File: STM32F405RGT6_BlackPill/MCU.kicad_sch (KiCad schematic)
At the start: 31 parts, among them J1 Conn_01x04, U1 STM32F405RGTx, Y1 25Mhz, Y2 Crystal

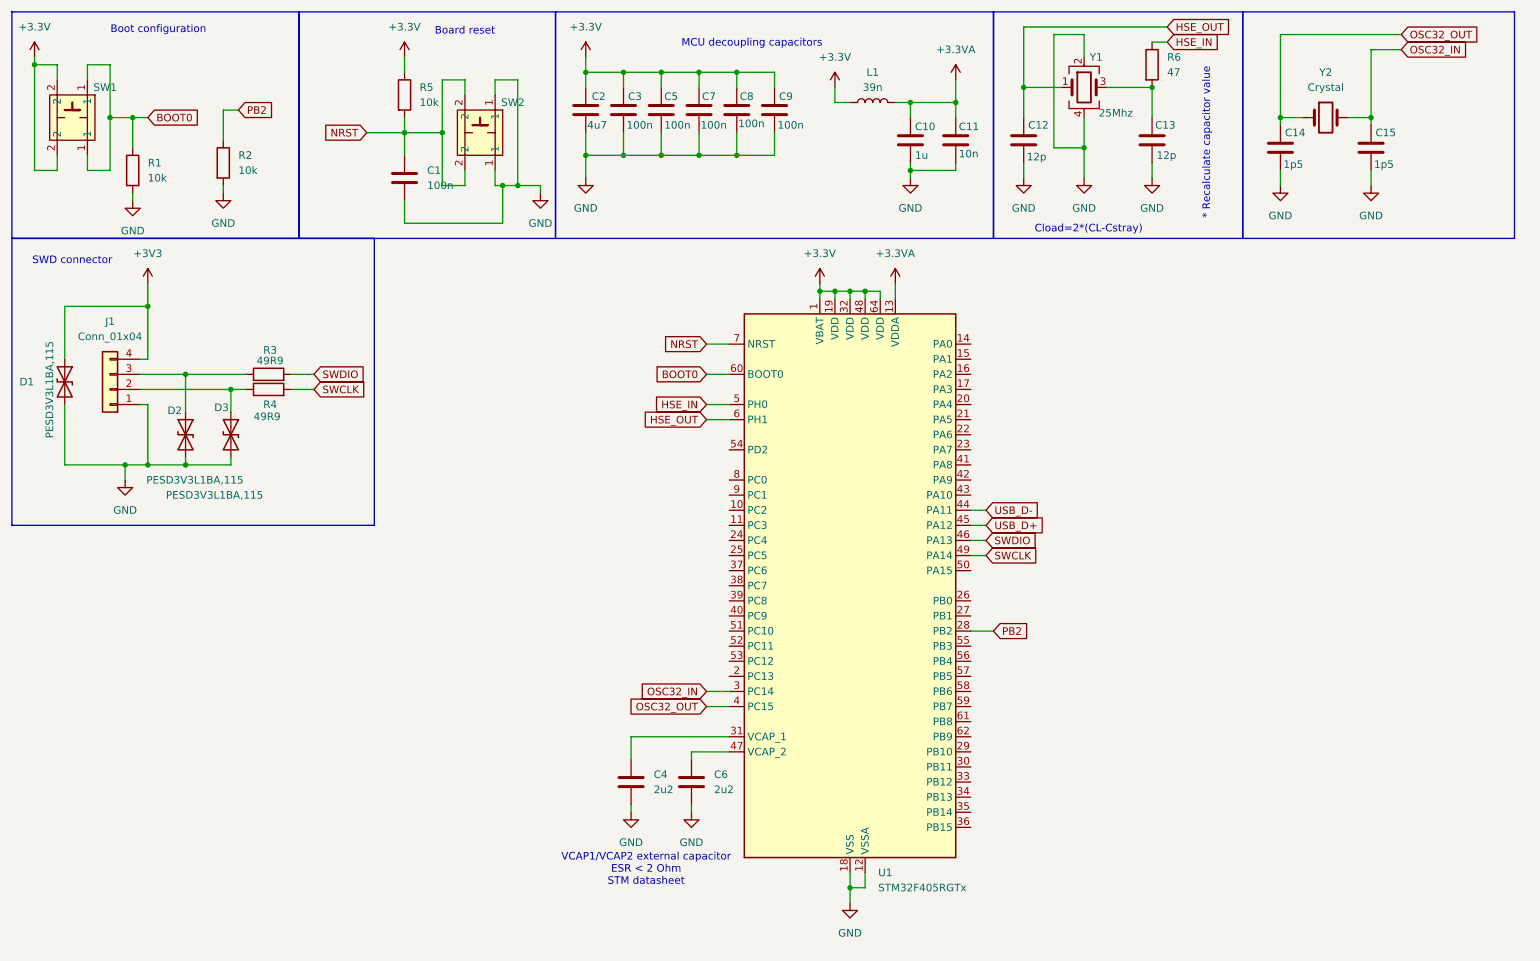
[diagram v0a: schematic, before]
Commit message: First version of the scheme
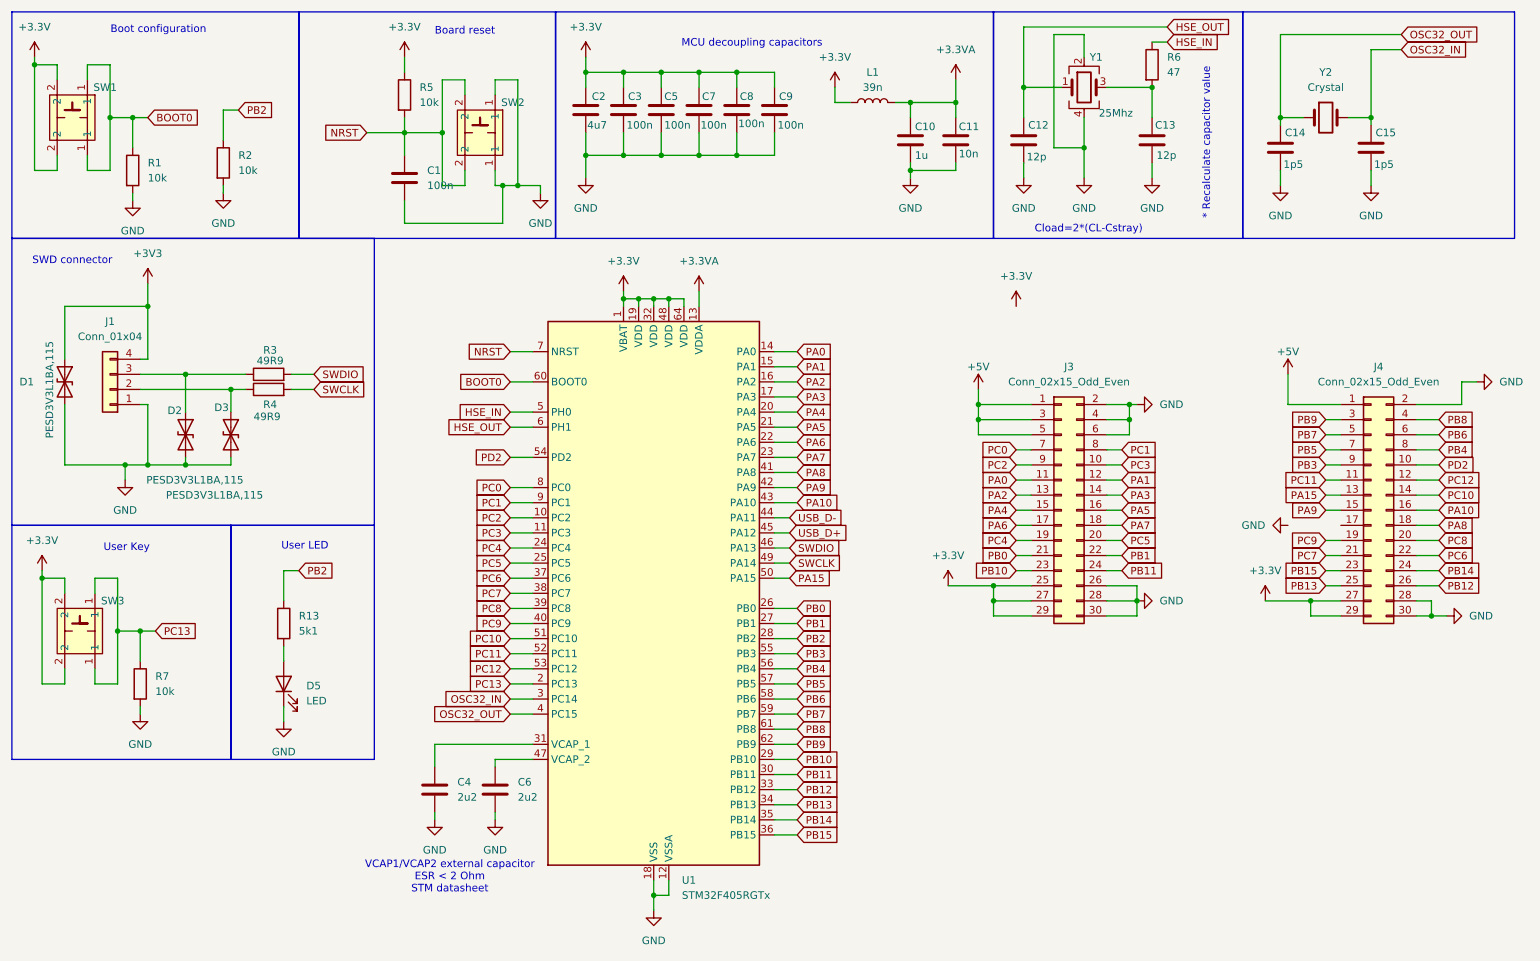
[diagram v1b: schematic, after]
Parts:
- added D5: LED, symbol Device:LED
- added J3, J4: Conn_02x15_Odd_Even, Connector_PinHeader_2.54mm:PinHeader_2x15_P2.54mm_Vertical, symbol Connector_Generic:Conn_02x15_Odd_Even
- added R13: 5k1, symbol Device:R
- added R7: 10k, symbol Device:R
- added SW3: ~, symbol BlackPillLibrary:SW_PUSH_6mm_H5mm
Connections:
- net +3.3V: now also J3.25 (Pin_25), J3.27 (Pin_27), J3.29 (Pin_29), J4.27 (Pin_27), J4.29 (Pin_29), SW3.2
- net GND: now also D5.1 (K), J3.2 (Pin_2), J3.26 (Pin_26), J3.28 (Pin_28), J3.30 (Pin_30), J3.4 (Pin_4), J3.6 (Pin_6), J4.2 (Pin_2), J4.28 (Pin_28), J4.30 (Pin_30), R7.2
- net PB2: now also R13.1
- net PC2: now reaches U1.10 (PC2)
- net PC2: now also J3.9 (Pin_9)
- net PC3: now reaches U1.11 (PC3)
- net PC3: now also J3.10 (Pin_10)
- net PA0: now reaches U1.14 (PA0)
- net PA0: now also J3.11 (Pin_11)
- net PA1: now reaches U1.15 (PA1)
- net PA1: now also J3.12 (Pin_12)
- net PA2: now reaches U1.16 (PA2)
- net PA2: now also J3.13 (Pin_13)
- net PA3: now reaches U1.17 (PA3)
- net PA3: now also J3.14 (Pin_14)
- net PC13: now reaches U1.2 (PC13)
- net PC13: now also R7.1, SW3.1
- net PA4: now reaches U1.20 (PA4)
- net PA4: now also J3.15 (Pin_15)
- net PA5: now reaches U1.21 (PA5)
- net PA5: now also J3.16 (Pin_16)
- net PA6: now reaches U1.22 (PA6)
- net PA6: now also J3.17 (Pin_17)
- net PA7: now reaches U1.23 (PA7)
- net PA7: now also J3.18 (Pin_18)
- net PC4: now reaches U1.24 (PC4)
- net PC4: now also J3.19 (Pin_19)
- net PC5: now reaches U1.25 (PC5)
- net PC5: now also J3.20 (Pin_20)
- net PB0: now reaches U1.26 (PB0)
- net PB0: now also J3.21 (Pin_21)
- net PB1: now reaches U1.27 (PB1)
- net PB1: now also J3.22 (Pin_22)
- net PB10: now reaches U1.29 (PB10)
- net PB10: now also J3.23 (Pin_23)
- net PB11: now reaches U1.30 (PB11)
- net PB11: now also J3.24 (Pin_24)
- net PB12: now reaches U1.33 (PB12)
- net PB12: now also J4.26 (Pin_26)
- net PB13: now reaches U1.34 (PB13)
- net PB13: now also J4.25 (Pin_25)
- net PB14: now reaches U1.35 (PB14)
- net PB14: now also J4.24 (Pin_24)
- net PB15: now reaches U1.36 (PB15)
- net PB15: now also J4.23 (Pin_23)
- net PC6: now reaches U1.37 (PC6)
- net PC6: now also J4.22 (Pin_22)
- net PC7: now reaches U1.38 (PC7)
- net PC7: now also J4.21 (Pin_21)
- net PC8: now reaches U1.39 (PC8)
- net PC8: now also J4.20 (Pin_20)
- net PC9: now reaches U1.40 (PC9)
- net PC9: now also J4.19 (Pin_19)
- net PA8: now reaches U1.41 (PA8)
- net PA8: now also J4.18 (Pin_18)
- net PA9: now reaches U1.42 (PA9)
- net PA9: now also J4.15 (Pin_15)
- net PA10: now reaches U1.43 (PA10)
- net PA10: now also J4.16 (Pin_16)
- net PA15: now reaches U1.50 (PA15)
- net PA15: now also J4.13 (Pin_13)
- net PC10: now reaches U1.51 (PC10)
- net PC10: now also J4.14 (Pin_14)
- net PC11: now reaches U1.52 (PC11)
- net PC11: now also J4.11 (Pin_11)
- net PC12: now reaches U1.53 (PC12)
- net PC12: now also J4.12 (Pin_12)
- net PD2: now reaches U1.54 (PD2)
- net PD2: now also J4.10 (Pin_10)
- net PB3: now reaches U1.55 (PB3)
- net PB3: now also J4.9 (Pin_9)
- net PB4: now reaches U1.56 (PB4)
- net PB4: now also J4.8 (Pin_8)
- net PB5: now reaches U1.57 (PB5)
- net PB5: now also J4.7 (Pin_7)
- net PB6: now reaches U1.58 (PB6)
- net PB6: now also J4.6 (Pin_6)
- net PB7: now reaches U1.59 (PB7)
- net PB7: now also J4.5 (Pin_5)
- net PB8: now reaches U1.61 (PB8)
- net PB8: now also J4.4 (Pin_4)
- net PB9: now reaches U1.62 (PB9)
- net PB9: now also J4.3 (Pin_3)
- net PC0: now reaches U1.8 (PC0)
- net PC0: now also J3.7 (Pin_7)
- net PC1: now reaches U1.9 (PC1)
- net PC1: now also J3.8 (Pin_8)
- new net: D5.2 (A), R13.2
- new net +5V: J3.1 (Pin_1), J3.3 (Pin_3), J3.5 (Pin_5), J4.1 (Pin_1)
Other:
- note added: "User Key"
- note added: "User LED"
- moved on the sheet: C4, C6, U1
